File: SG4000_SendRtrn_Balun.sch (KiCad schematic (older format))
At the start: 40 parts, among them J1001 Power Entry, J1002 Audio to MB, J1003 Audio To XLR, U1001 NE5532AP, U1002 NE5534AP

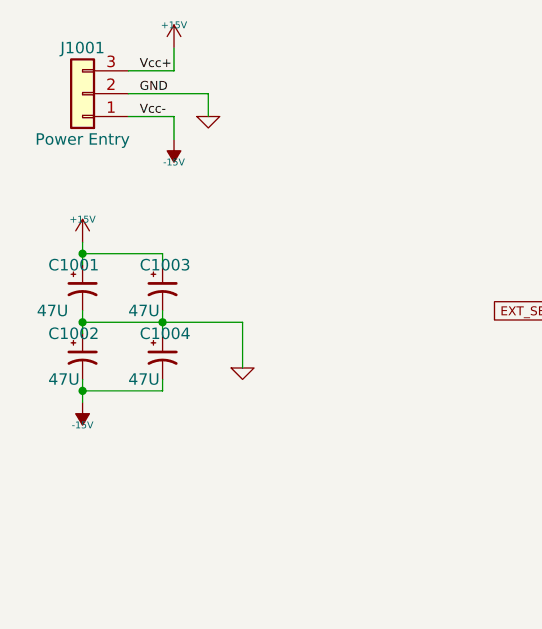
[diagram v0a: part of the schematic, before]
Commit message: Add files via upload
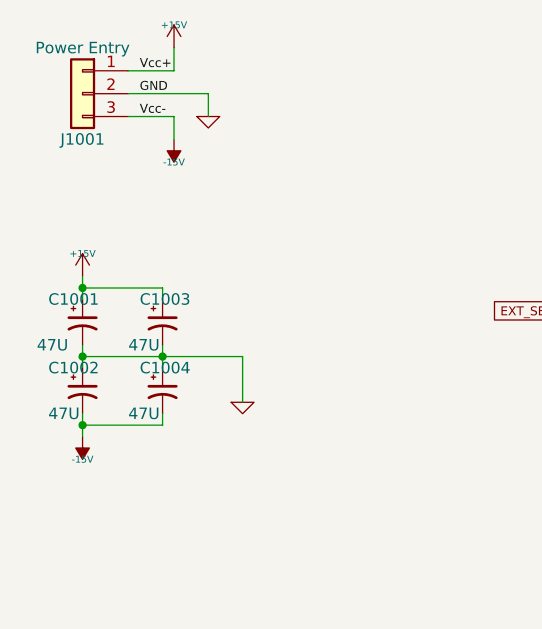
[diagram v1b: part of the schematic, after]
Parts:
- C1001, C1002, C1003, C1004: footprint (none) -> Capacitors_THT:CP_Radial_D6.3mm_P2.50mm
- C1005, C1008, C1009, C1010, C1013, C1014, C1020, C1022: footprint (none) -> Capacitors_THT:C_Rect_L7.2mm_W4.5mm_P5.00mm_FKS2_FKP2_MKS2_MKP2
- C1006, C1007, C1018: footprint (none) -> Capacitors_THT:CP_Radial_D5.0mm_P2.00mm
- C1011, C1012, C1015, C1016, C1017: footprint (none) -> Capacitors_THT:C_Rect_L4.0mm_W2.5mm_P2.50mm
- C1019, C1021: footprint (none) -> Capacitors_THT:CP_Radial_D8.0mm_P3.50mm
- J1001: footprint (none) -> Pin_Headers:Pin_Header_Straight_1x03_Pitch2.54mm
- J1002: footprint (none) -> Pin_Headers:Pin_Header_Straight_1x04_Pitch2.54mm
- J1003: footprint (none) -> Pin_Headers:Pin_Header_Straight_1x05_Pitch2.54mm
- R1001, R1002, R1003, R1004, R1005, R1006, R1007, R1008, R1009, R1010, R1011, R1012, R1013: footprint (none) -> Resistors_THT:R_Axial_DIN0207_L6.3mm_D2.5mm_P10.16mm_Horizontal
- U1001, U1002: footprint (none) -> Housings_DIP:DIP-8_W7.62mm
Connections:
- net +15V: now also J1001.1 (Pin_1); no longer J1001.3 (Pin_3)
- net -15V: now also J1001.3 (Pin_3); no longer J1001.1 (Pin_1)
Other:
- moved on the sheet: C1001, C1002, C1003, C1004
